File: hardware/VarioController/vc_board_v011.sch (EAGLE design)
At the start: 50 parts, among them IC1 WeMos D1 mini, IC2 MP2016DJ, IC3 DS3502U+, X1 SPTAF_1/3_3,5, X2 SPTAF_1/3_3,5, X3 SPTAF_1/3_3,5, X4 SPTAF_1/8_3,5, X5 05-JST-B5B-XH-A, X6 03-JST-B3B-XH-A

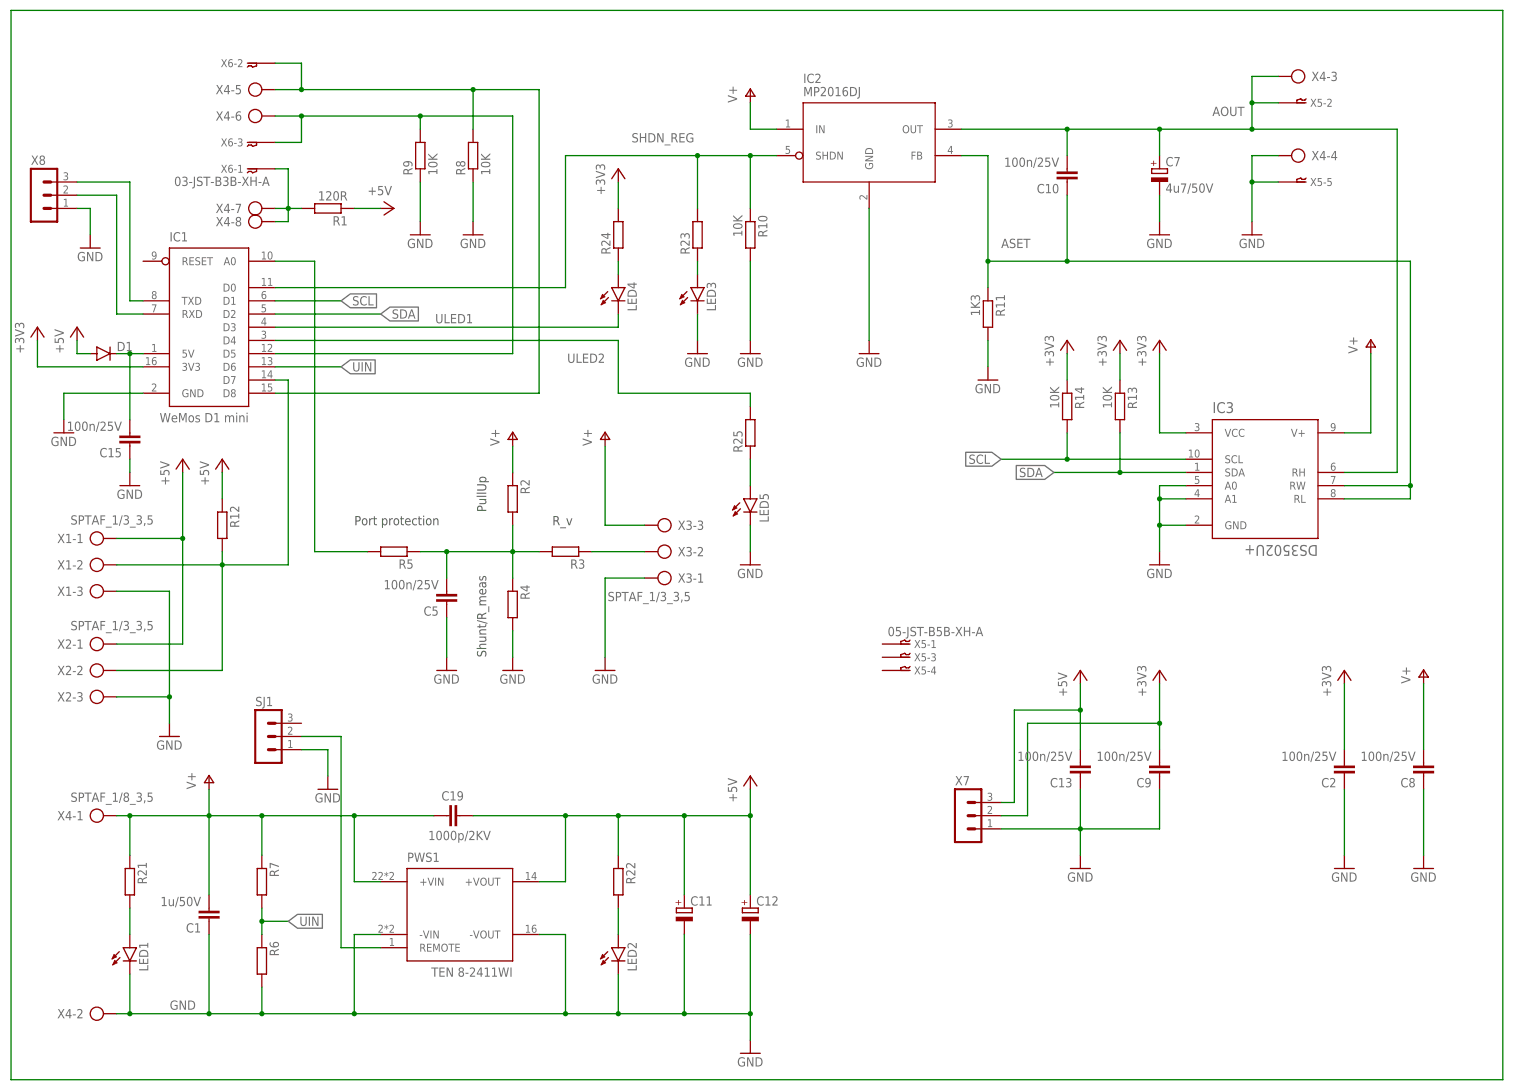
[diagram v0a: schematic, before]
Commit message: Update values
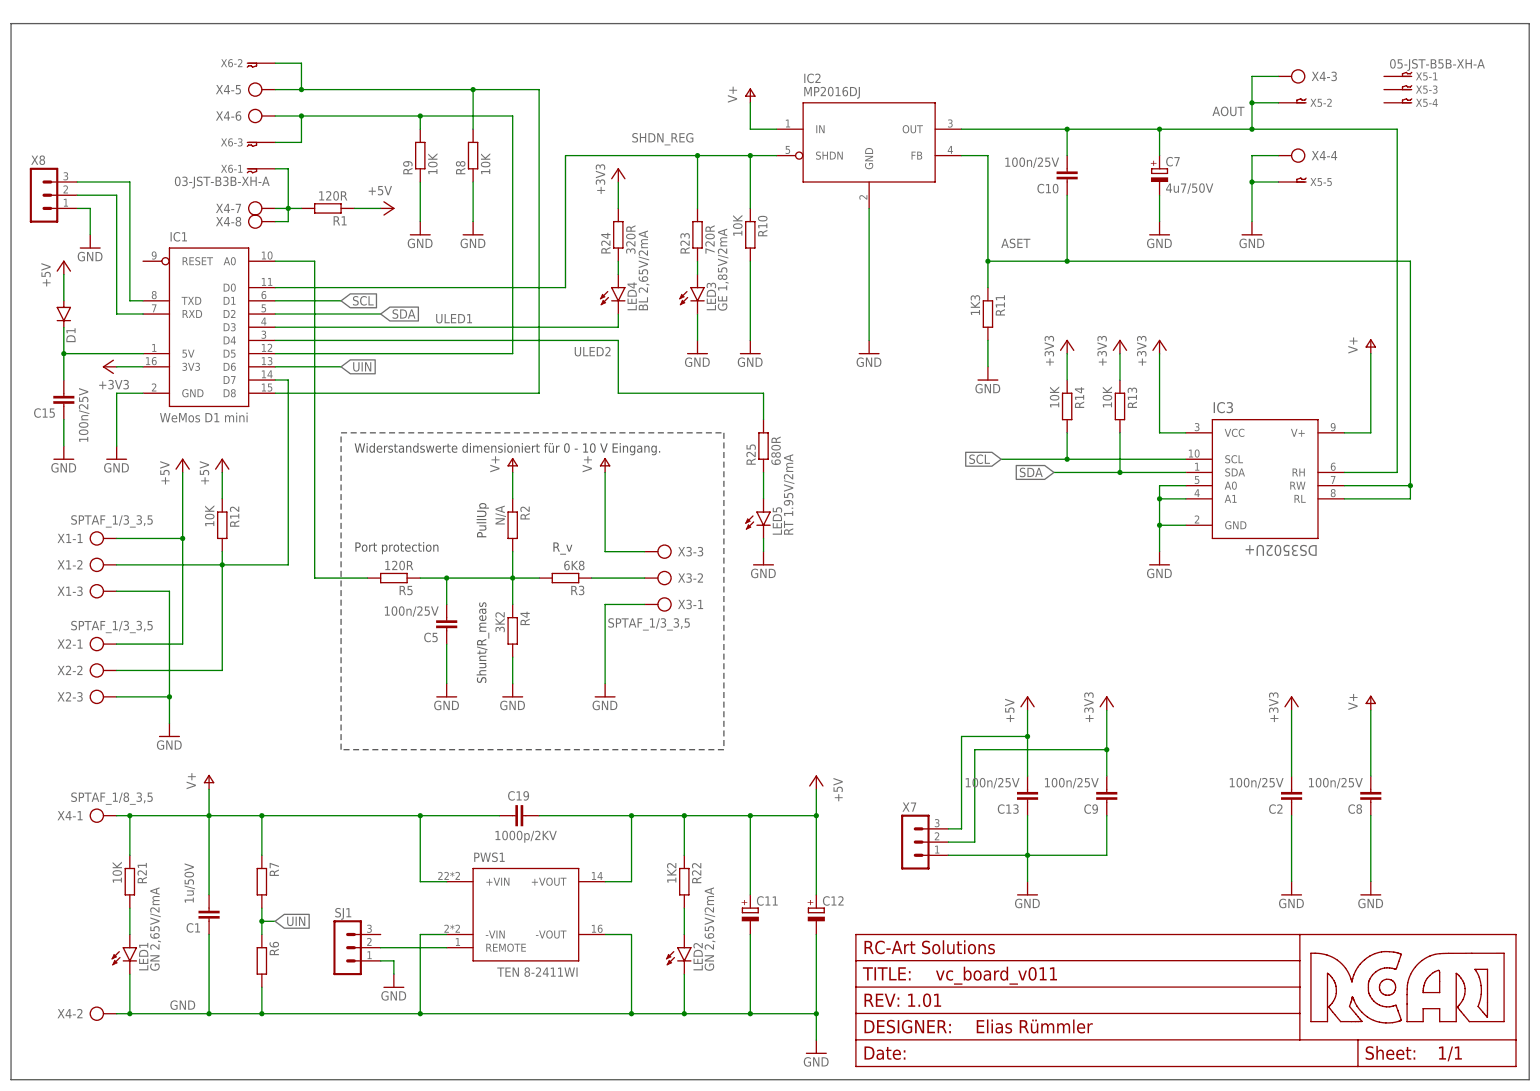
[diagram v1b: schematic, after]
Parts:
- added FRAME1: MF_FRAMEDEFAULT, rca-frames:MF_FRAMEDEFAULT
- LED1, LED2: value (none) -> GN 2,65V/2mA; FARNELL_SKU (none) -> 2846598
- LED3: value (none) -> GE 1,85V/2mA; FARNELL_SKU (none) -> 2846596
- LED4: value (none) -> BL 2,65V/2mA; FARNELL_SKU (none) -> 2846594
- LED5: value (none) -> RT 1.95V/2mA; FARNELL_SKU (none) -> 2099241
- R12, R21: value (none) -> 10K
- R2: value (none) -> N/A
- R22: value (none) -> 1K2
- R23: value (none) -> 720R
- R24: value (none) -> 320R
- R25: value (none) -> 680R
- R3: value (none) -> 6K8
- R4: value (none) -> 3K2
- R5: value (none) -> 120R
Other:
- note added: "Widerstandswerte dimensioniert für 0 - 10 V Eingang."
- moved on the sheet: C11, C12, C13, C15, C19, C2, C5, C8, C9, D1, LED2, LED5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
